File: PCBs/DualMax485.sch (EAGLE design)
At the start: 14 parts, among them IC2 7805DT, J1 6V-12V

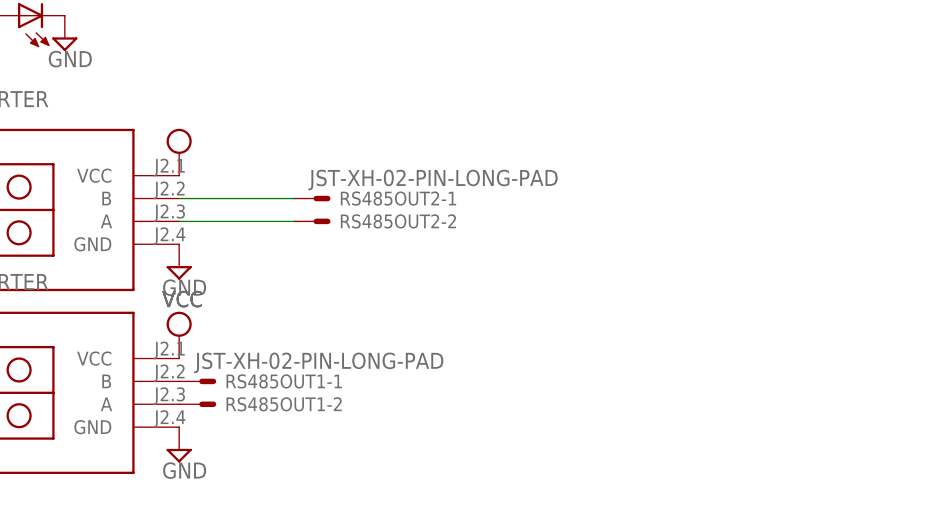
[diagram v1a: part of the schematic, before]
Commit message: updated board
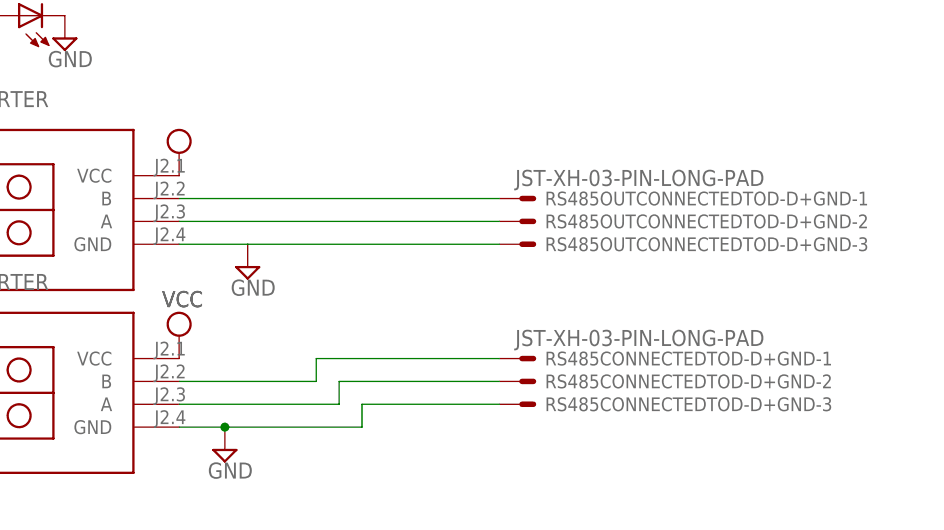
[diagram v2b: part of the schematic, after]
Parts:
- removed RS485OUT1, RS485OUT2: JST-XH-02-PIN-LONG-PAD, Rembrandt Electronics - JST XH Connectors v1-0:JST-XH-02-PIN-LONG-PAD
- added RS485CONNECTEDTOD-D+GND, RS485OUTCONNECTEDTOD-D+GND: JST-XH-03-PIN-LONG-PAD, Rembrandt Electronics - JST XH Connectors v1-0:JST-XH-03-PIN-LONG-PAD
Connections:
- net GND: now also RS485CONNECTEDTOD-D+GND-3.S, RS485OUTCONNECTEDTOD-D+GND-3.S
- net N$12: now also RS485CONNECTEDTOD-D+GND-1.S; no longer RS485OUT1-1.S
- net N$13: now also RS485CONNECTEDTOD-D+GND-2.S; no longer RS485OUT1-2.S
- net N$4: now also RS485OUTCONNECTEDTOD-D+GND-1.S; no longer RS485OUT2-1.S
- net N$6: now also RS485OUTCONNECTEDTOD-D+GND-2.S; no longer RS485OUT2-2.S
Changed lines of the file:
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@@
 <part name="RS232IN" library="Rembrandt Electronics - JST XH Connectors v1-0" deviceset="JST-XH-07-PIN" device="-LONG-PAD"/>
 <part name="SUPPLY17" library="supply2" library_urn="urn:adsk.eagle:library:372" deviceset="GND" device=""/>
-<part name="RS485OUT1" library="Rembrandt Electronics - JST XH Connectors v1-0" deviceset="JST-XH-02-PIN" device="-LONG-PAD"/>
-<part name="RS485OUT2" library="Rembrandt Electronics - JST XH Connectors v1-0" deviceset="JST-XH-02-PIN" device="-LONG-PAD"/>
 <part name="IC2" library="adafruit" deviceset="78*" device="DT" technology="05"/>
 <part name="RS485MODULE2" library="diy-modules" deviceset="RS485-TTL-CONVERTER" device=""/>
@@
 <part name="R4" library="adafruit" deviceset="R-US_" device="M0805" value="1k"/>
 <part name="R5" library="adafruit" deviceset="R-US_" device="M0805" value="1k"/>
+<part name="RS485OUTCONNECTEDTOD-D+GND" library="Rembrandt Electronics - JST XH Connectors v1-0" deviceset="JST-XH-03-PIN" device="-LONG-PAD"/>
+<part name="RS485CONNECTEDTOD-D+GND" library="Rembrandt Electronics - JST XH Connectors v1-0" deviceset="JST-XH-03-PIN" device="-LONG-PAD"/>
 </parts>
 <sheets>
@@
 <attribute name="VALUE" x="-24.765" y="89.535" size="1.778" layer="96"/>
 </instance>
-<instance part="SUPPLY6" gate="GND" x="-22.86" y="73.66" smashed="yes">
-<attribute name="VALUE" x="-24.765" y="70.485" size="1.778" layer="96"/>
+<instance part="SUPPLY6" gate="GND" x="-17.78" y="73.66" smashed="yes">
+<attribute name="VALUE" x="-19.685" y="70.485" size="1.778" layer="96"/>
 </instance>
 <instance part="SUPPLY12" gate="GND" x="-83.82" y="127" smashed="yes" rot="R180">
@@
 <attribute name="VALUE" x="-24.765" y="89.535" size="1.778" layer="96"/>
 </instance>
-<instance part="SUPPLY3" gate="GND" x="-22.86" y="93.98" smashed="yes">
-<attribute name="VALUE" x="-24.765" y="90.805" size="1.778" layer="96"/>
+<instance part="SUPPLY3" gate="GND" x="-15.24" y="93.98" smashed="yes">
+<attribute name="VALUE" x="-17.145" y="90.805" size="1.778" layer="96"/>
 </instance>
 <instance part="SUPPLY1" gate="G$1" x="-96.52" y="116.84" smashed="yes" rot="R90">
@@
 <attribute name="VALUE" x="-70.485" y="85.725" size="1.778" layer="96"/>
 </instance>
-<instance part="RS485OUT1" gate="-2" x="-20.32" y="78.74" smashed="yes">
-<attribute name="NAME" x="-17.78" y="77.978" size="1.524" layer="95"/>
-</instance>
-<instance part="RS485OUT1" gate="-1" x="-20.32" y="81.28" smashed="yes">
-<attribute name="NAME" x="-17.78" y="80.518" size="1.524" layer="95"/>
-<attribute name="VALUE" x="-21.082" y="82.677" size="1.778" layer="96"/>
-</instance>
-<instance part="RS485OUT2" gate="-2" x="-7.62" y="99.06" smashed="yes">
-<attribute name="NAME" x="-5.08" y="98.298" size="1.524" layer="95"/>
-</instance>
-<instance part="RS485OUT2" gate="-1" x="-7.62" y="101.6" smashed="yes">
-<attribute name="NAME" x="-5.08" y="100.838" size="1.524" layer="95"/>
-<attribute name="VALUE" x="-8.382" y="102.997" size="1.778" layer="96"/>
-</instance>
 <instance part="IC2" gate="A1" x="-83.82" y="116.84" smashed="yes" rot="R180">
 <attribute name="NAME" x="-76.2" y="111.125" size="1.778" layer="95" rot="R180"/>
@@
 <attribute name="NAME" x="-82.55" y="72.6186" size="1.778" layer="95"/>
 <attribute name="VALUE" x="-82.55" y="67.818" size="1.778" layer="96"/>
+</instance>
+<instance part="RS485OUTCONNECTEDTOD-D+GND" gate="-1" x="15.24" y="101.6" smashed="yes">
+<attribute name="NAME" x="17.78" y="100.838" size="1.524" layer="95"/>
+<attribute name="VALUE" x="14.478" y="102.997" size="1.778" layer="96"/>
+</instance>
+<instance part="RS485OUTCONNECTEDTOD-D+GND" gate="-2" x="15.24" y="99.06" smashed="yes">
+<attribute name="NAME" x="17.78" y="98.298" size="1.524" layer="95"/>
+</instance>
+<instance part="RS485OUTCONNECTEDTOD-D+GND" gate="-3" x="15.24" y="96.52" smashed="yes">
+<attribute name="NAME" x="17.78" y="95.758" size="1.524" layer="95"/>
+</instance>
+<instance part="RS485CONNECTEDTOD-D+GND" gate="-1" x="15.24" y="83.82" smashed="yes">
+<attribute name="NAME" x="17.78" y="83.058" size="1.524" layer="95"/>
+<attribute name="VALUE" x="14.478" y="85.217" size="1.778" layer="96"/>
+</instance>
+<instance part="RS485CONNECTEDTOD-D+GND" gate="-2" x="15.24" y="81.28" smashed="yes">
+<attribute name="NAME" x="17.78" y="80.518" size="1.524" layer="95"/>
+</instance>
+<instance part="RS485CONNECTEDTOD-D+GND" gate="-3" x="15.24" y="78.74" smashed="yes">
+<attribute name="NAME" x="17.78" y="77.978" size="1.524" layer="95"/>
 </instance>
 </instances>
@@
 <pinref part="RS485MODULE2" gate="G$1" pin="GND"/>
 <pinref part="SUPPLY3" gate="GND" pin="GND"/>
+<pinref part="RS485OUTCONNECTEDTOD-D+GND" gate="-3" pin="S"/>
+<wire x1="-15.24" y1="96.52" x2="12.7" y2="96.52" width="0.1524" layer="91"/>
+<wire x1="-15.24" y1="96.52" x2="-22.86" y2="96.52" width="0.1524" layer="91"/>
 </segment>
 <segment>
 <pinref part="RS485MODULE1" gate="G$1" pin="GND"/>
 <pinref part="SUPPLY6" gate="GND" pin="GND"/>
+<wire x1="-17.78" y1="76.2" x2="-2.54" y2="76.2" width="0.1524" layer="91"/>
+<wire x1="-2.54" y1="76.2" x2="-2.54" y2="78.74" width="0.1524" layer="91"/>
+<pinref part="RS485CONNECTEDTOD-D+GND" gate="-3" pin="S"/>
+<wire x1="-2.54" y1="78.74" x2="12.7" y2="78.74" width="0.1524" layer="91"/>
+<wire x1="-17.78" y1="76.2" x2="-22.86" y2="76.2" width="0.1524" layer="91"/>
+<junction x="-17.78" y="76.2"/>
 </segment>
 </net>
@@
 <segment>
 <pinref part="RS485MODULE2" gate="G$1" pin="B"/>
-<pinref part="RS485OUT2" gate="-1" pin="S"/>
-<wire x1="-10.16" y1="101.6" x2="-22.86" y2="101.6" width="0.1524" layer="91"/>
+<wire x1="-22.86" y1="101.6" x2="12.7" y2="101.6" width="0.1524" layer="91"/>
+<pinref part="RS485OUTCONNECTEDTOD-D+GND" gate="-1" pin="S"/>
 </segment>
 </net>
@@
 <segment>
 <pinref part="RS485MODULE2" gate="G$1" pin="A"/>
-<pinref part="RS485OUT2" gate="-2" pin="S"/>
-<wire x1="-10.16" y1="99.06" x2="-22.86" y2="99.06" width="0.1524" layer="91"/>
+<pinref part="RS485OUTCONNECTEDTOD-D+GND" gate="-2" pin="S"/>
+<wire x1="-22.86" y1="99.06" x2="12.7" y2="99.06" width="0.1524" layer="91"/>
 </segment>
 </net>
@@
 <net name="N$12" class="0">
 <segment>
+<pinref part="RS485CONNECTEDTOD-D+GND" gate="-1" pin="S"/>
+<wire x1="-7.62" y1="83.82" x2="12.7" y2="83.82" width="0.1524" layer="91"/>
+<wire x1="-7.62" y1="81.28" x2="-7.62" y2="83.82" width="0.1524" layer="91"/>
 <pinref part="RS485MODULE1" gate="G$1" pin="B"/>
-<pinref part="RS485OUT1" gate="-1" pin="S"/>
+<wire x1="-22.86" y1="81.28" x2="-7.62" y2="81.28" width="0.1524" layer="91"/>
 </segment>
 </net>
@@
 <segment>
 <pinref part="RS485MODULE1" gate="G$1" pin="A"/>
-<pinref part="RS485OUT1" gate="-2" pin="S"/>
-</segment>
-</net>
+<wire x1="-22.86" y1="78.74" x2="-5.08" y2="78.74" width="0.1524" layer="91"/>
+<wire x1="-5.08" y1="78.74" x2="-5.08" y2="81.28" width="0.1524" layer="91"/>
+<pinref part="RS485CONNECTEDTOD-D+GND" gate="-2" pin="S"/>
+<wire x1="-5.08" y1="81.28" x2="12.7" y2="81.28" width="0.1524" layer="91"/>
+</segment>
+</net>

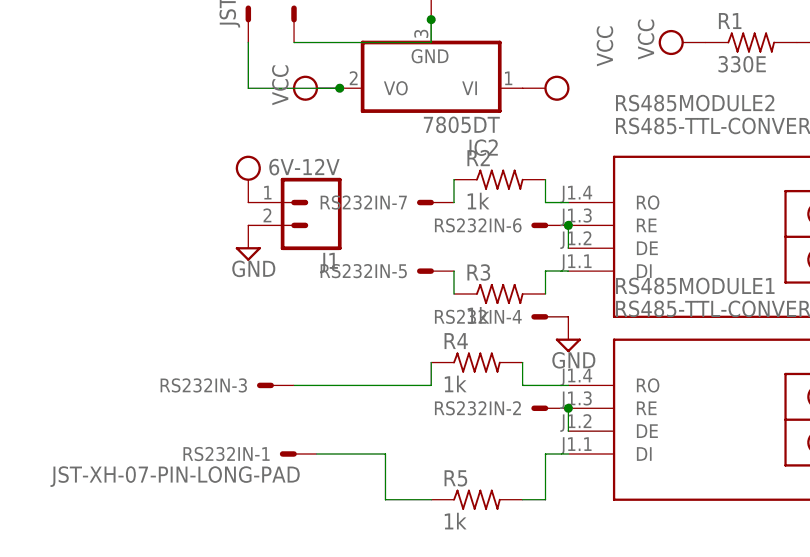
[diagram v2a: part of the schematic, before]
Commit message: board updated
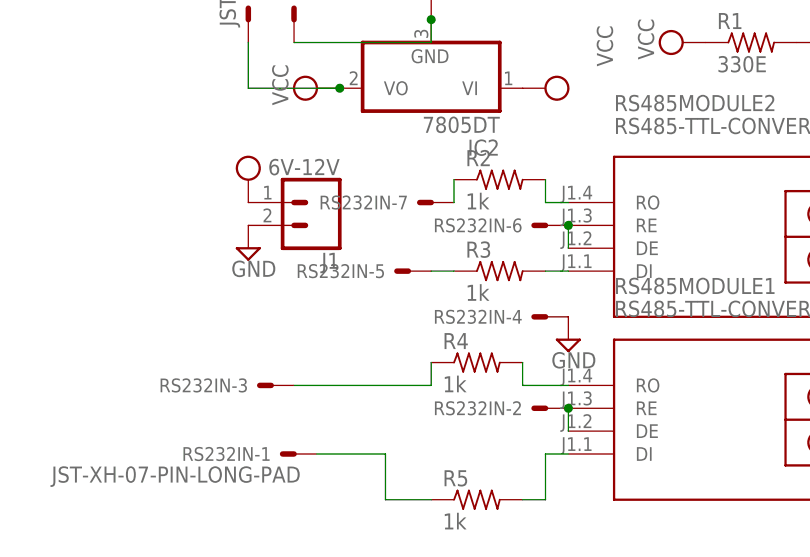
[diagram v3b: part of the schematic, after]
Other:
- moved on the sheet: R3, RS232IN-5
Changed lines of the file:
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@@
 <attribute name="NAME" x="-73.66" y="92.202" size="1.524" layer="95" rot="R180"/>
 </instance>
-<instance part="RS232IN" gate="-5" x="-83.82" y="96.52" smashed="yes" rot="R180">
-<attribute name="NAME" x="-86.36" y="97.282" size="1.524" layer="95" rot="R180"/>
+<instance part="RS232IN" gate="-5" x="-86.36" y="96.52" smashed="yes" rot="R180">
+<attribute name="NAME" x="-88.9" y="97.282" size="1.524" layer="95" rot="R180"/>
 </instance>
 <instance part="RS232IN" gate="-6" x="-71.12" y="101.6" smashed="yes" rot="R180">
@@
 <attribute name="VALUE" x="-80.01" y="103.378" size="1.778" layer="96"/>
 </instance>
-<instance part="R3" gate="G$1" x="-76.2" y="93.98" smashed="yes">
-<attribute name="NAME" x="-80.01" y="95.4786" size="1.778" layer="95"/>
-<attribute name="VALUE" x="-80.01" y="90.678" size="1.778" layer="96"/>
+<instance part="R3" gate="G$1" x="-76.2" y="96.52" smashed="yes">
+<attribute name="NAME" x="-80.01" y="98.0186" size="1.778" layer="95"/>
+<attribute name="VALUE" x="-80.01" y="93.218" size="1.778" layer="96"/>
 </instance>
 <instance part="R4" gate="G$1" x="-78.74" y="86.36" smashed="yes">
@@
 <pinref part="R3" gate="G$1" pin="2"/>
 <wire x1="-71.12" y1="96.52" x2="-68.58" y2="96.52" width="0.1524" layer="91"/>
-<wire x1="-71.12" y1="96.52" x2="-71.12" y2="93.98" width="0.1524" layer="91"/>
 </segment>
 </net>
@@
 <pinref part="R3" gate="G$1" pin="1"/>
 <pinref part="RS232IN" gate="-5" pin="S"/>
-<wire x1="-81.28" y1="96.52" x2="-81.28" y2="93.98" width="0.1524" layer="91"/>
-</segment>
-</net>
+<wire x1="-83.82" y1="96.52" x2="-81.28" y2="96.52" width="0.1524" layer="91"/>
+</segment>
+</net>
